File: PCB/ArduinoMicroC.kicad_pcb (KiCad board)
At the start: 4 copper layers, 18 x 36.2 mm, 28 parts, among them J1 USB_C_Receptacle_USB2.0, J2 Conn_01x12, J3 Conn_01x06, J4 Conn_01x12, SW1 SW_Check_USB, SW2 SW_Push, U1 MIC5219-5.0YM5, U2 ATmega32U4-MU, Y1 16MHz

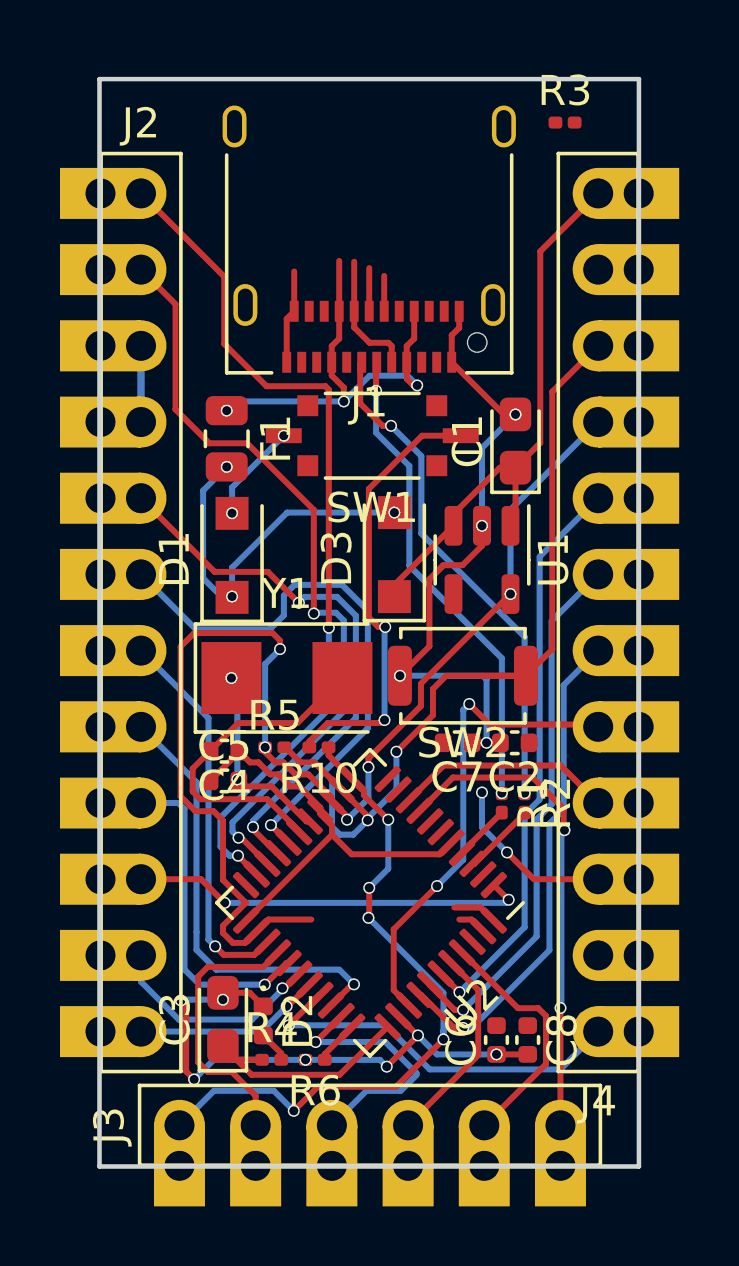
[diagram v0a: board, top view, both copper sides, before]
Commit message: First version of PCB
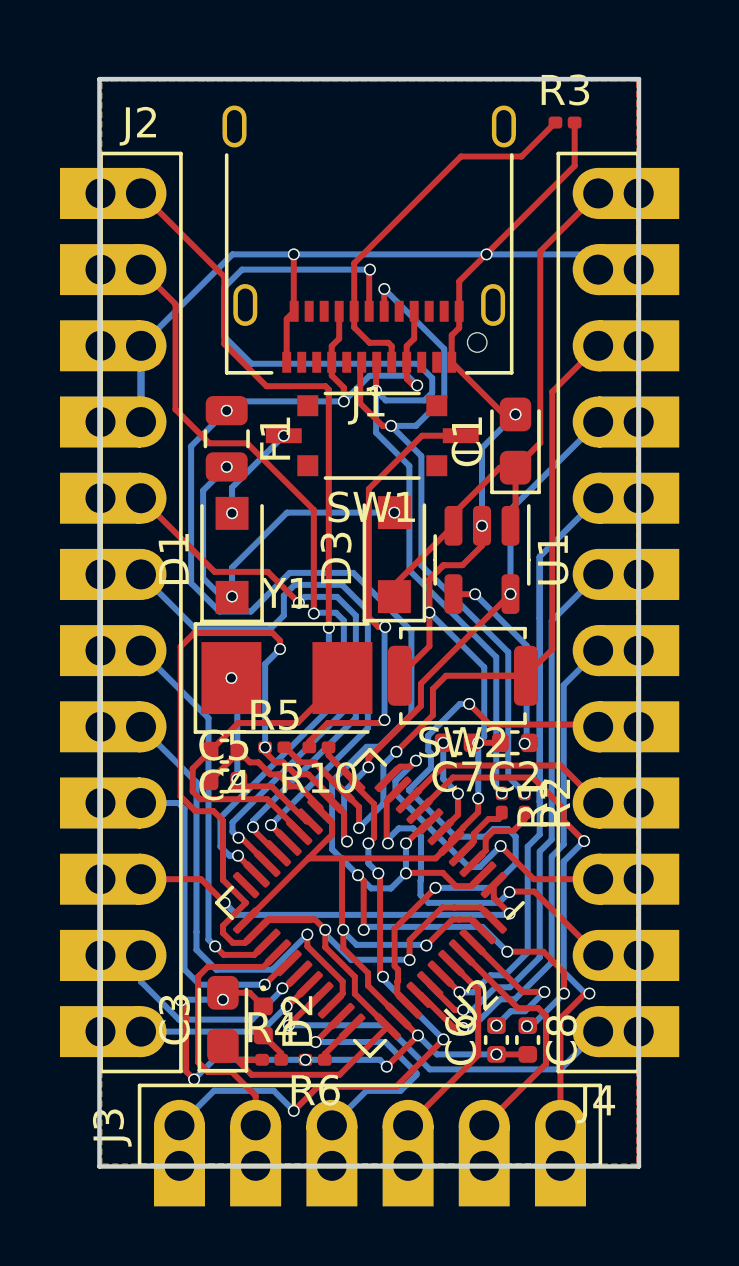
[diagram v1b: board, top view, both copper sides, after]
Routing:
- net VBUS: track 14.7 -> 56.9 mm, vias 3 -> 10
- net GND: track 65.8 -> 106.1 mm, vias 11 -> 16
- net Net-(J1-PadA6): track 17.6 -> 34.5 mm, vias 2 -> 3
- net VCC: track 53.5 -> 66.8 mm, vias 5 -> 7
- net MOSI: track 0.96 -> 13.4 mm, vias 0 -> 2
- net A3: track 20.2 -> 29.0 mm
- net Net-(J1-PadA5): track 4.24 -> 12.8 mm
- net Net-(C2-Pad1): track 0.00 -> 6.60 mm, vias 0 -> 2
- net Net-(J1-PadA7): track 18.0 -> 24.2 mm, vias 2 -> 3
- net A0: track 17.1 -> 22.8 mm
- net MISO: track 6.71 -> 12.1 mm
- net AREF: track 0.00 -> 5.15 mm, vias 0 -> 2
- net Net-(C7-Pad2): track 0.00 -> 3.42 mm, vias 0 -> 2
- net RESET: track 28.9 -> 26.4 mm
- net SS: track 17.3 -> 18.7 mm
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- added copper zone on B.Cu, net GND
- added copper zone on F.Cu, net GND
